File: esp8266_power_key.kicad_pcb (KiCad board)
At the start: 2 copper layers, 25 parts, among them P1 CONN_01X06, P2 CONN_01X06, Q1 Q_PMOS_GDS, Q2 Q_PMOS_GDS, Q3 BC849, Q4 BC849, U1 ESP-01v090, U2 LP2988AIMX-3.3/NOPB

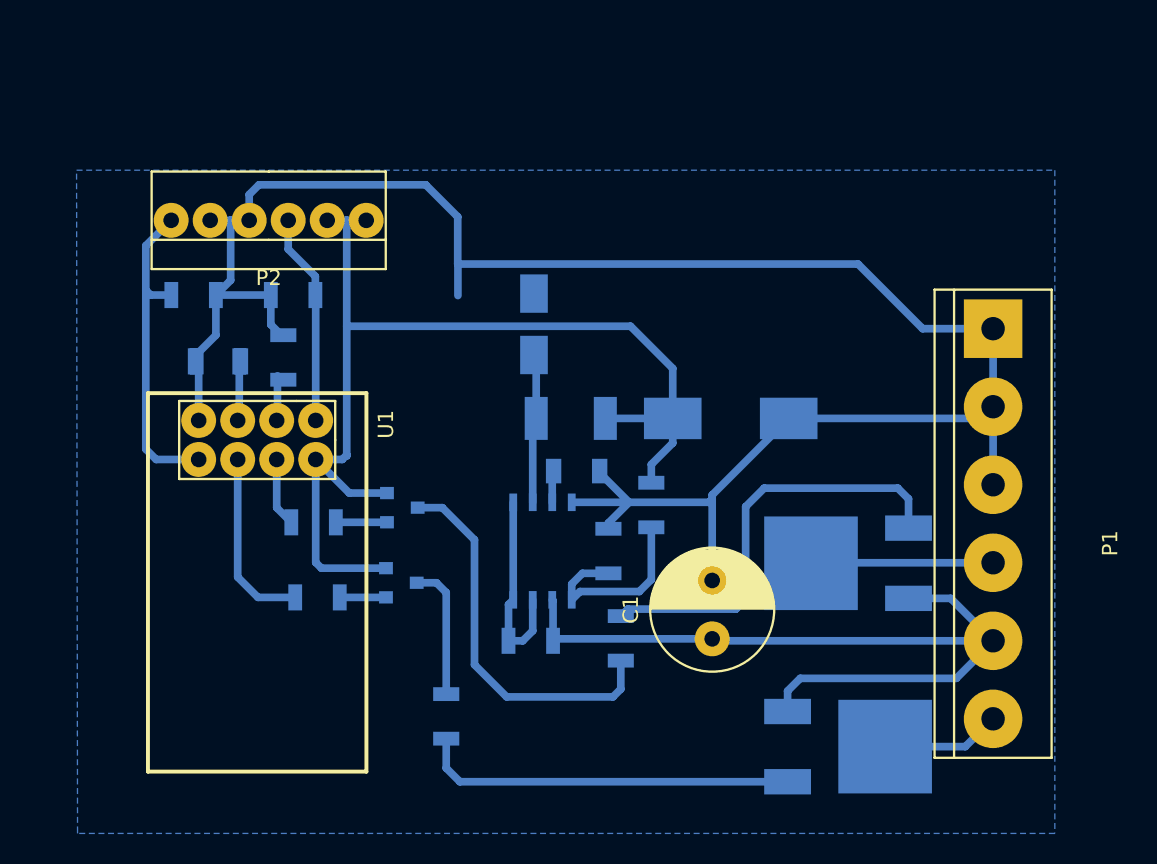
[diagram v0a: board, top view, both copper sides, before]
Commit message: changed size
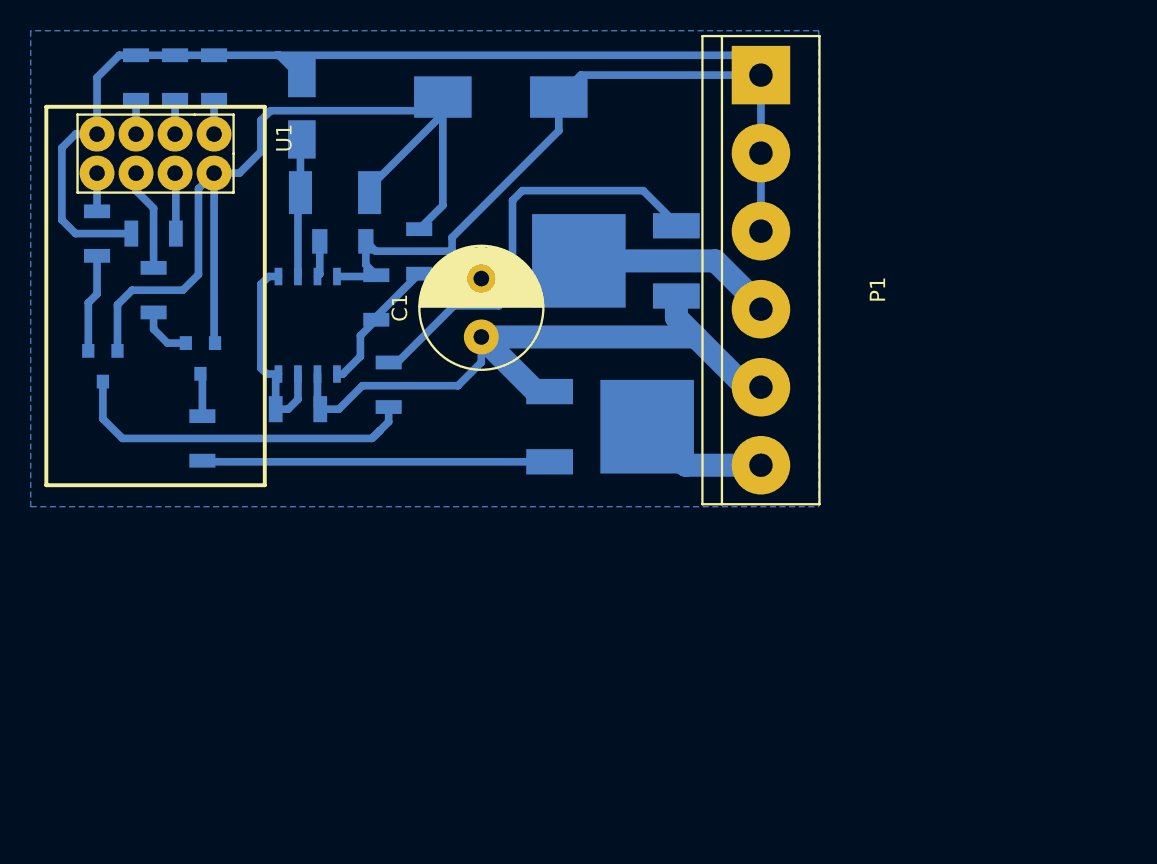
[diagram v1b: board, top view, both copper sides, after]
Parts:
- removed P2: CONN_01X06, Connect:PINHEAD1-6
- removed the R2 at (29.1, 33.7)
- moved Q1 26.0 mm to (50.7, 38.0)
- moved C2 25.7 mm to (47.5, 16.5)
- moved Q2 24.8 mm to (58.9, 27.2)
- moved C1 24.7 mm to (46.2, 32.1)
- moved R4 24.1 mm to (28.1, 38.7)
- moved R10 23.5 mm to (21.2, 25.4), turned to 270 degrees
- moved R9 22.7 mm to (24.9, 29.1), turned to 270 degrees
- moved P1 22.4 mm to (64.4, 27.8)
- moved R11 22.4 mm to (39.4, 29.6)
- moved R5 22.4 mm to (40.2, 35.2)
- moved R7 22.4 mm to (42.2, 26.6)
- moved Q4 21.6 mm to (21.6, 34.0), turned to 270 degrees
- moved R6 21.4 mm to (34.3, 36.8)
- moved C3 21.3 mm to (37.2, 25.9)
- moved L1 21.3 mm to (36.7, 22.7)
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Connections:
- R8 pad 2: Net-(P2-Pad6) -> Net-(R8-Pad2)
- U1 pad 4: Net-(R10-Pad1) -> Net-(R8-Pad2)
- U1 pad 8: Net-(P2-Pad6) -> Net-(R10-Pad1)
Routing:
- net Net-(P2-Pad6): track 21.3 -> 0.00 mm
- net GND: track 131.6 -> 115.2 mm
- net Net-(R1-Pad1): track 13.8 -> 2.23 mm
- net Net-(C1-Pad1): track 55.9 -> 44.4 mm
- net Net-(C2-Pad2): track 71.8 -> 64.0 mm
- net Net-(Q3-Pad3): track 8.80 -> 2.81 mm
- net Net-(R9-Pad1): track 11.9 -> 6.64 mm
- net Net-(R8-Pad2): track 0.00 -> 3.96 mm
- net Net-(R11-Pad2): track 12.8 -> 8.97 mm
- net Net-(Q4-Pad1): track 3.33 -> 6.42 mm
- net Net-(R10-Pad1): track 4.48 -> 2.49 mm
- net Net-(Q1-Pad1): track 24.5 -> 22.6 mm
- net Net-(R2-Pad1): track 3.89 -> 2.23 mm
- net Net-(Q4-Pad3): track 25.2 -> 23.5 mm
- net Net-(P1-Pad4): track 11.9 -> 13.3 mm
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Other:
- net class pwr added: clearance 0.2, trace_width 1.5, via_dia 0.6, via_drill 0.4
